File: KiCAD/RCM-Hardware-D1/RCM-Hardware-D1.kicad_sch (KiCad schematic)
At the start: 2 parts, among them U1 WeMos_D1_mini, U2 L293D

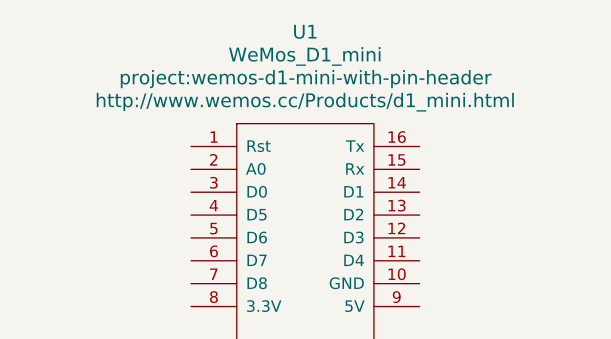
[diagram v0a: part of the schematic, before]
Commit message: set up kicad
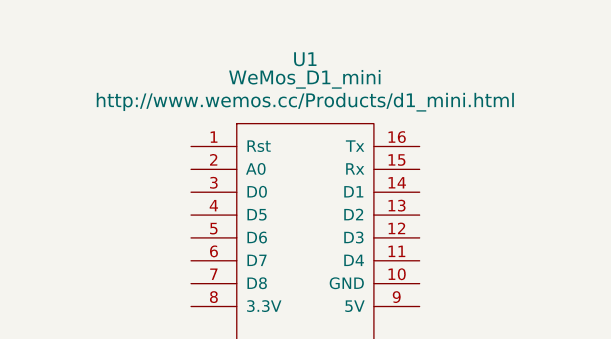
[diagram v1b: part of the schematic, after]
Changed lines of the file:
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@@
 		(on_board yes)
 		(dnp no)
-		(fields_autoplaced yes)
 		(property "Reference" "U1"
-			(at 106.68 38.1 0)
+			(at 106.68 41.148 0)
 			(effects
 				(font
@@
 		)
 		(property "Value" "WeMos_D1_mini"
-			(at 106.68 40.64 0)
+			(at 106.68 43.18 0)
 			(effects
 				(font
@@
 					(size 1.524 1.524)
 				)
+				(hide yes)
 			)
 		)
